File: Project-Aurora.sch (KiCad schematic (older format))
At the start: 54 parts, among them P1 USB_OTG, P2 FLASH_HDR, SW1 Reset, U1 IS31FL3732, U2 Freescale_K20P64M72SF1, U3 TPS62086, U5 IS31FL3732, U6 Case-Ground, X1 CRYSTAL_SMD

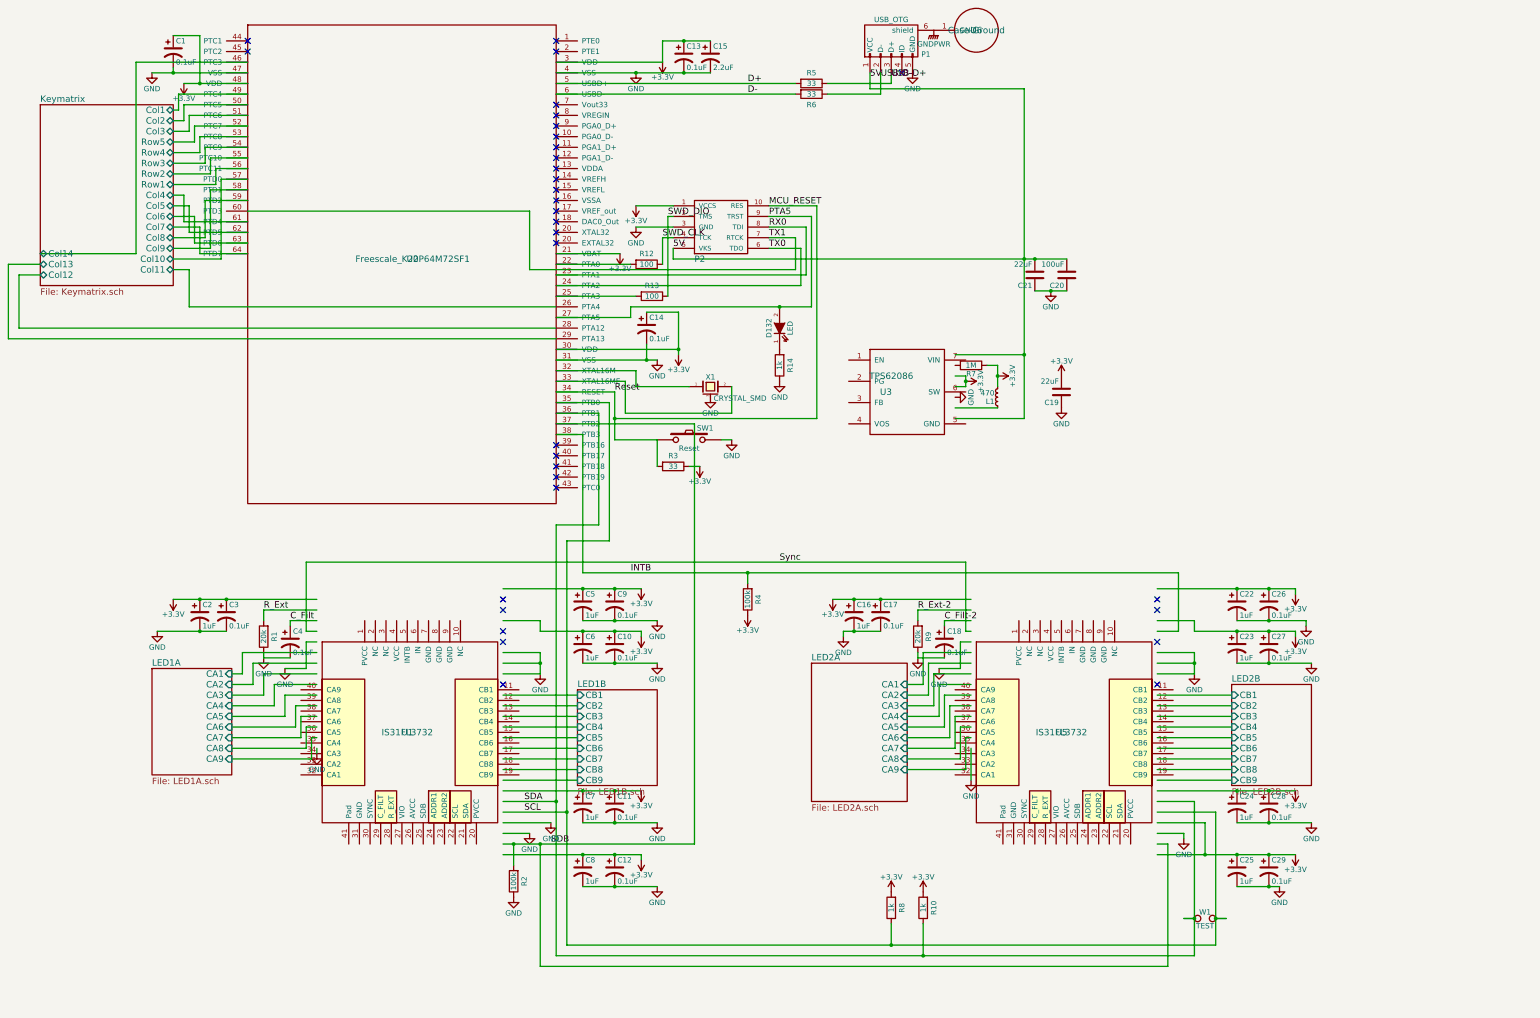
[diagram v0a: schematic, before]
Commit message: Forgot some Stuff in the last Commit
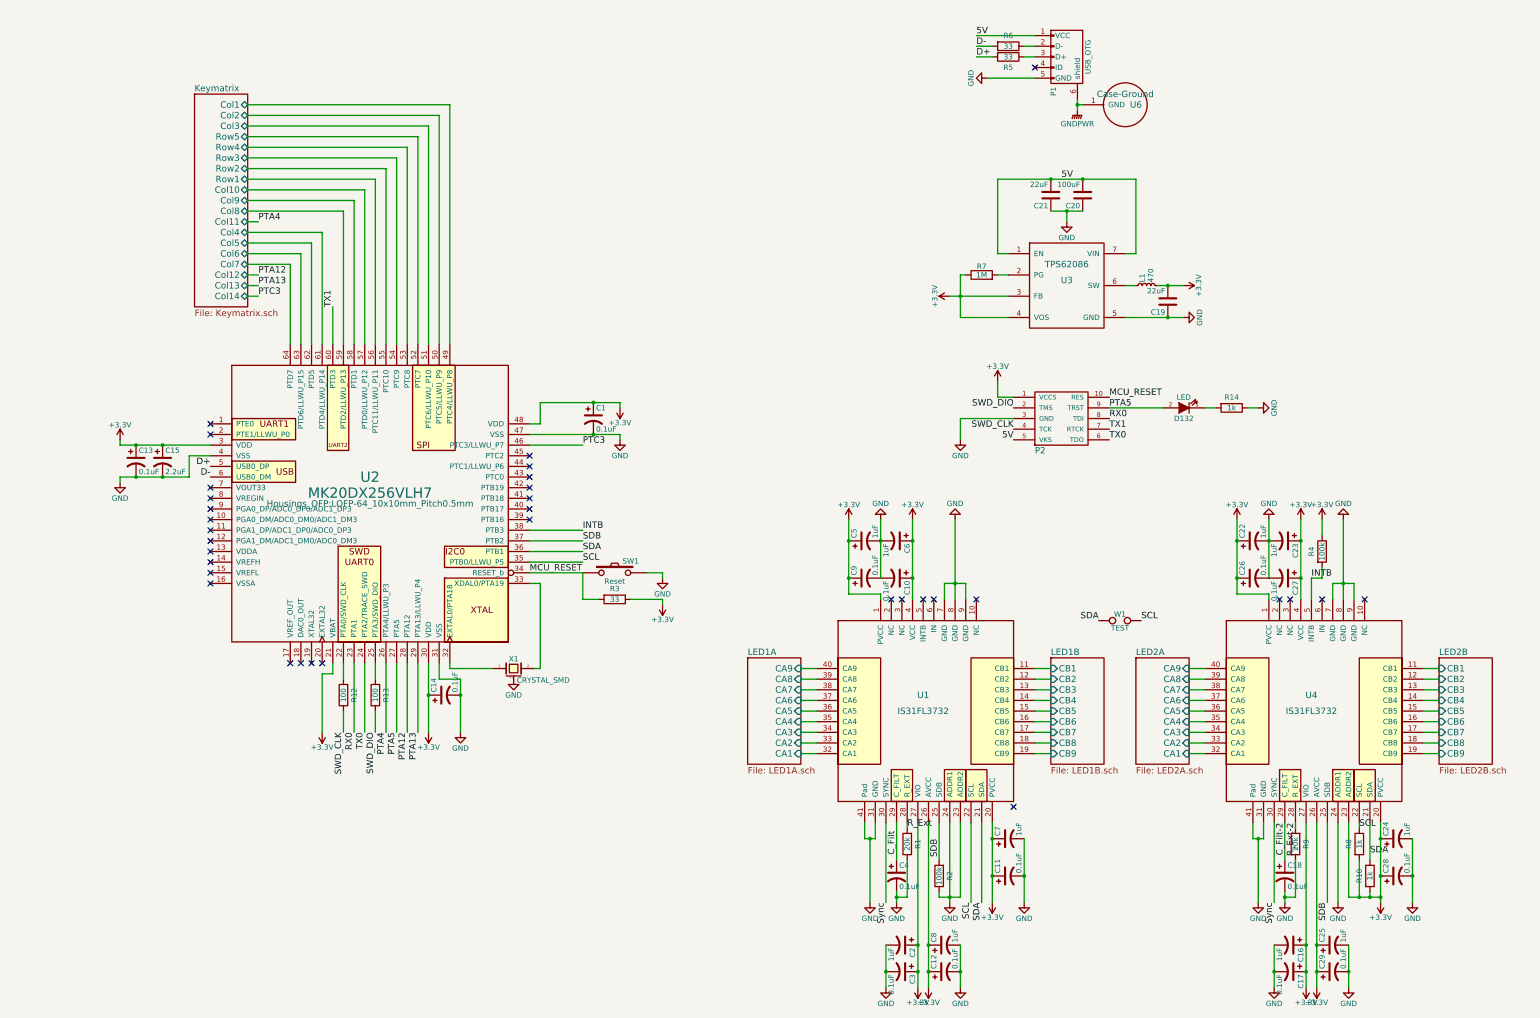
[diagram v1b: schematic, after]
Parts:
- removed U2: Freescale_K20P64M72SF1, Housings_QFP:LQFP-64_10x10mm_Pitch0.5mm, symbol Freescale_K20P64M72SF1
- removed U5: IS31FL3732, Housings_DFN_QFN:UQFN-40-1EP_5x5mm_Pitch0.4mm, symbol IS31FL3732
- added U2: MK20DX256VLH7, Housings_QFP:LQFP-64_10x10mm_Pitch0.5mm, symbol MK20DX256VLH7
- added U4: IS31FL3732, Housings_DFN_QFN:UQFN-40-1EP_5x5mm_Pitch0.4mm, symbol IS31FL3732
- P2: footprint mx2a:JLINK_NEEDLE -> Keyboard_Stuff:JLINK_NEEDLE
- SW1: footprint mx2a:KSEM31GLFS -> Keyboard_Stuff:KSEM31GLFS
- U3: footprint mx2a:VSON-7 -> Keyboard_Stuff:VSON-7
- U6: footprint mx2a:PKRHC -> Keyboard_Stuff:PKRHC
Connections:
- net labels added: PTA12, PTA13, PTA4, PTC3
- net labels removed: Reset, USB-D+, USB-D-
- wire segments 307 -> 216
- no-connect marks 33 -> 34
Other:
- moved on the sheet: C1, C10, C11, C12, C13, C14, C15, C16, C17, C18, C19, C2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
